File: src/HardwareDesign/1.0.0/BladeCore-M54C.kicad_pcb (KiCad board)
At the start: 6 copper layers, 29 x 80.6 mm, 152 parts, among them IC1 RP2354B, IC2 AT24C256C-XHL-T, IC29 TCAN1044AVDRBRQ1, IC3 W25Q128JVPIQ, IC4 MCP6001RT, IC5 LM4040B30FTA, IC6 MCP2515T-I/ML, IC7 TPS74801DRCT, IC8 SN74LVC1G97QDCKRQ1, IC9 FSUSB42MUX, J1 MDT320M03001, J2 SM03B-SRSS-TB, J3 USB-TYPE-C-018, SW1 B3U-1000P, SW2 B3U-1000P, X1 12MHz 10pF, X2 16MHz 8pF

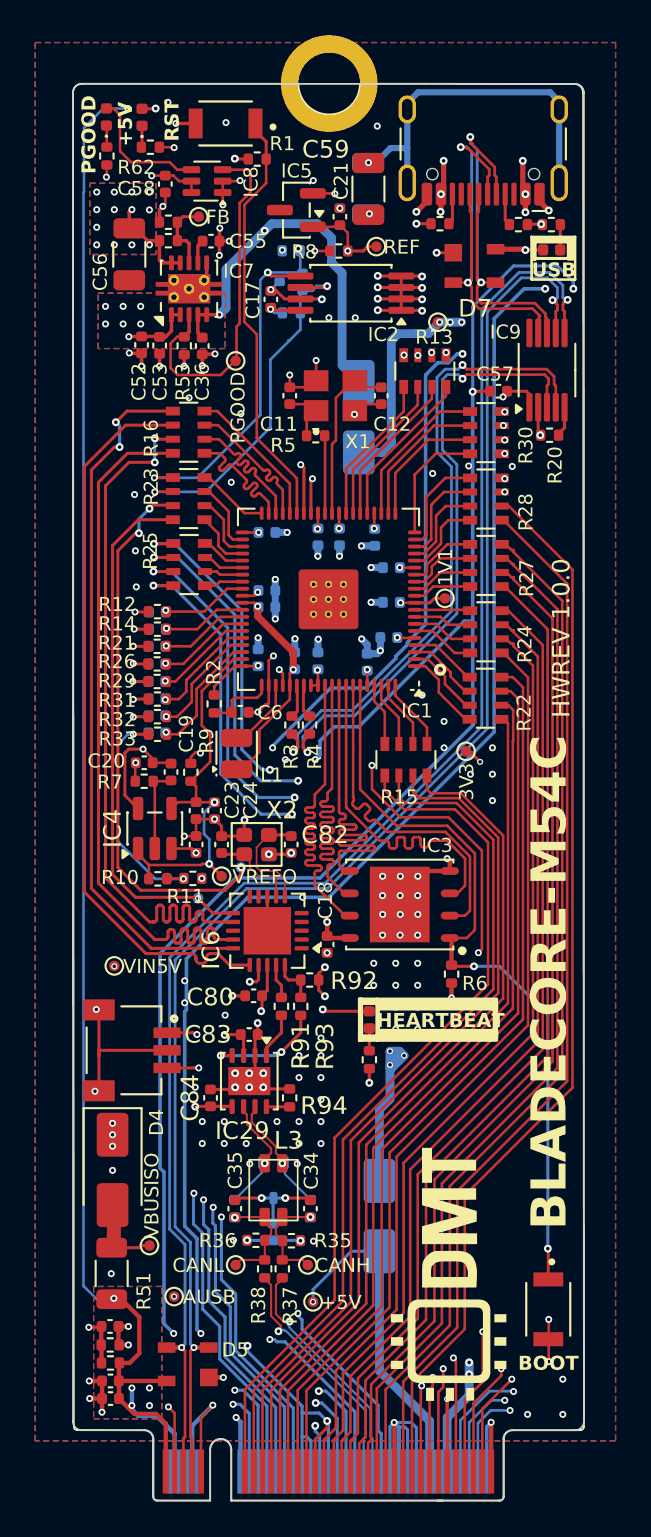
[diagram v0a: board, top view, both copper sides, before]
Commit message: update documentation
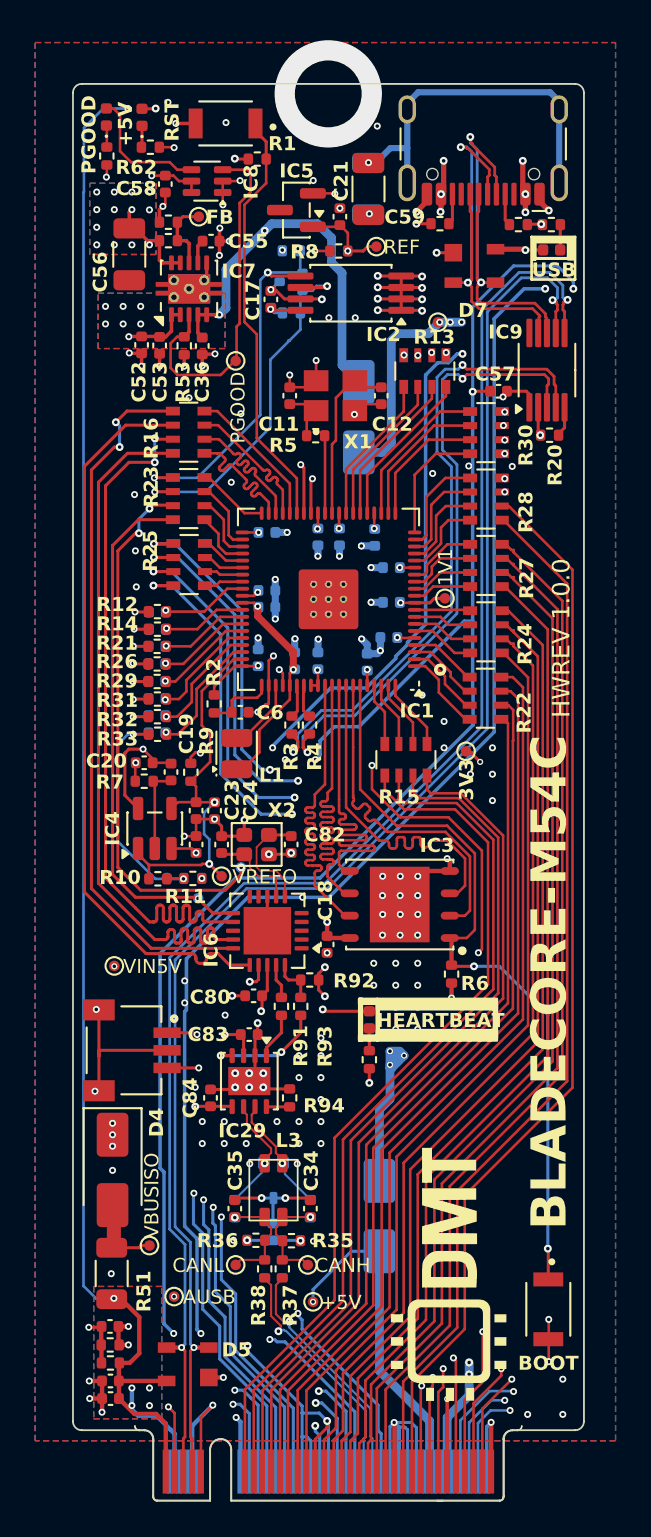
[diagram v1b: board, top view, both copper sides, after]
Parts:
- J1: footprint DS_Connector:M.2-M-KEY_Card_2280 -> DS_Connector:M.2-M-KEY_Card_Plain
- moved J1 39.1 mm to (221.4, 164.6)
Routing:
- net GND: vias 177 -> 178
